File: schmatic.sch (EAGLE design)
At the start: 18 parts, among them SW1 SWITCH-SMD-EVQP-P2602W

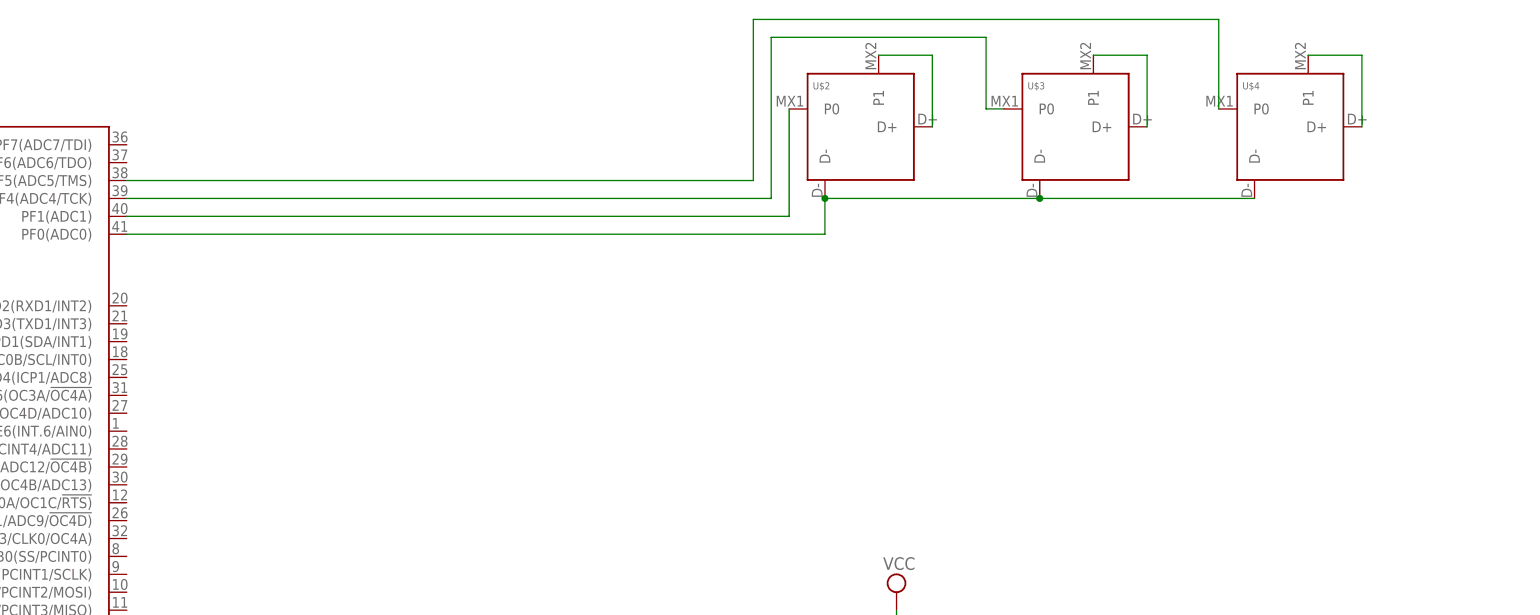
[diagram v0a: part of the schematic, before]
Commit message: updated based off feedback, included extra osh screenshot
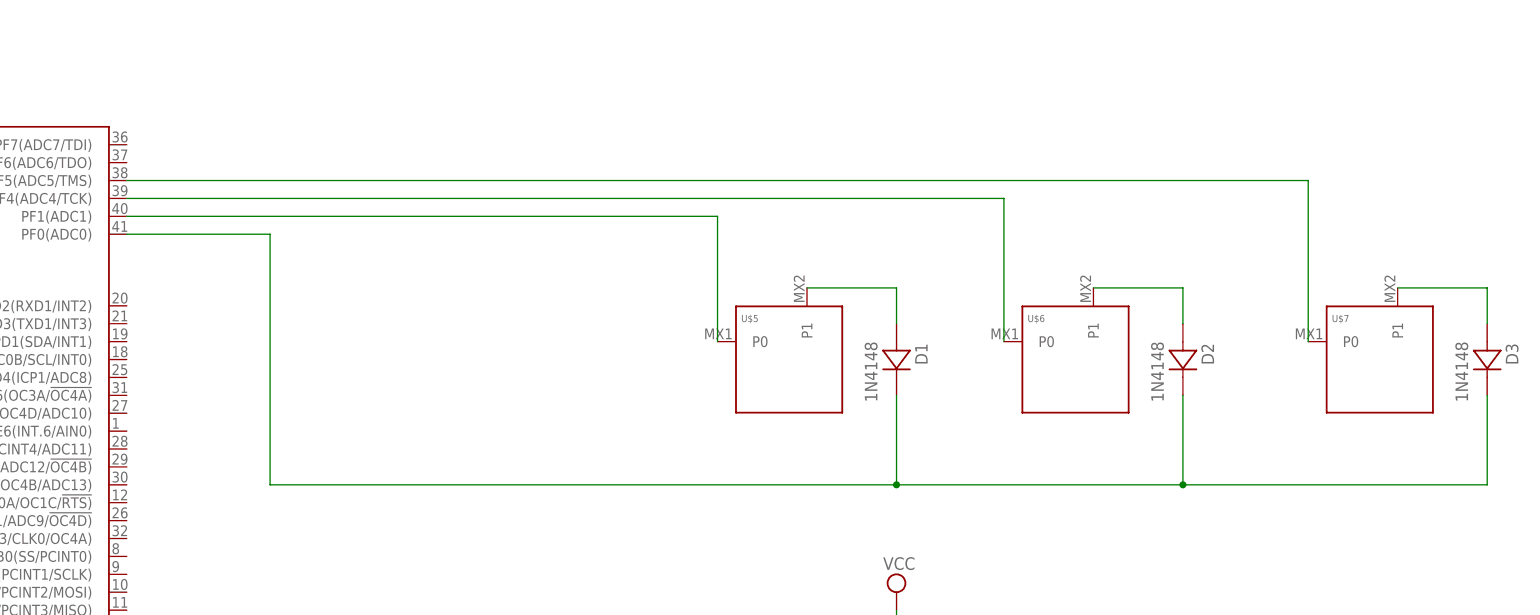
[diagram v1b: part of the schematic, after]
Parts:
- removed U$2, U$3, U$4: KEYSWITCH-DIODE-MX-1U-DIODE, Keyboard:KEYSWITCH-DIODE-MX-1U-DIODE
- added D1, D2, D3: 1N4148, Components:DIODE-DO-35
- added U$5, U$6, U$7: KEYSWITCH-PLAIN-MXHSPCB-1U, Keyboard:KEYSWITCH-PLAIN-MXHSPCB-1U
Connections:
- removed net N$11: U$3.D+, U$3.P1
- removed net N$12: U$4.D+, U$4.P1
- removed net N$16: U$1.PF5(ADC5/TMS), U$4.P0
- new net N$17: D1.A, U$5.P1
- new net N$18: D2.A, U$6.P1
- new net N$19: D3.A, U$7.P1
- net N$13: now also D1.C, D2.C, D3.C; no longer U$2.D-, U$3.D-, U$4.D-
- net N$14: now also U$5.P0; no longer U$2.P0
- net N$15: now also U$1.PF5(ADC5/TMS), U$7.P0; no longer U$1.PF4(ADC4/TCK), U$3.P0
- net N$9: now also U$1.PF4(ADC4/TCK), U$6.P0; no longer U$2.D+, U$2.P1
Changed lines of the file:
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@@
 <part name="SUPPLY6" library="supply2" library_urn="urn:adsk.eagle:library:372" deviceset="GND" device=""/>
 <part name="C8" library="Components" deviceset="CAPACITOR" device="-0402" value="1uF"/>
-<part name="U$2" library="Keyboard" deviceset="KEYSWITCH-DIODE" device="-MX-1U-DIODE"/>
-<part name="U$3" library="Keyboard" deviceset="KEYSWITCH-DIODE" device="-MX-1U-DIODE"/>
-<part name="U$4" library="Keyboard" deviceset="KEYSWITCH-DIODE" device="-MX-1U-DIODE"/>
 <part name="SUPPLY7" library="supply2" library_urn="urn:adsk.eagle:library:372" deviceset="GND" device=""/>
 <part name="SUPPLY8" library="supply2" library_urn="urn:adsk.eagle:library:372" deviceset="GND" device=""/>
@@
 <part name="SUPPLY14" library="supply2" library_urn="urn:adsk.eagle:library:372" deviceset="VCC" device=""/>
 <part name="SUPPLY15" library="supply2" library_urn="urn:adsk.eagle:library:372" deviceset="VCC" device=""/>
+<part name="U$5" library="Keyboard" deviceset="KEYSWITCH-PLAIN" device="-MXHSPCB-1U"/>
+<part name="U$6" library="Keyboard" deviceset="KEYSWITCH-PLAIN" device="-MXHSPCB-1U"/>
+<part name="U$7" library="Keyboard" deviceset="KEYSWITCH-PLAIN" device="-MXHSPCB-1U"/>
+<part name="D1" library="Components" deviceset="DIODE" device="-DO-35" value="1N4148"/>
+<part name="D2" library="Components" deviceset="DIODE" device="-DO-35" value="1N4148"/>
+<part name="D3" library="Components" deviceset="DIODE" device="-DO-35" value="1N4148"/>
 </parts>
 <sheets>
@@
 <attribute name="VALUE" x="77.216" y="86.106" size="1.778" layer="96" align="top-left"/>
 </instance>
-<instance part="U$2" gate="G$1" x="259.08" y="106.68" smashed="yes">
-<attribute name="NAME" x="252.27" y="111.998" size="1" layer="95"/>
-</instance>
-<instance part="U$3" gate="G$1" x="289.56" y="106.68" smashed="yes">
-<attribute name="NAME" x="282.75" y="111.998" size="1" layer="95"/>
-</instance>
-<instance part="U$4" gate="G$1" x="320.04" y="106.68" smashed="yes">
-<attribute name="NAME" x="313.23" y="111.998" size="1" layer="95"/>
-</instance>
 <instance part="SUPPLY7" gate="GND" x="93.98" y="38.1" smashed="yes" rot="R270">
 <attribute name="VALUE" x="90.805" y="40.005" size="1.778" layer="96" rot="R270"/>
@@
 <instance part="SUPPLY15" gate="G$1" x="93.98" y="91.44" smashed="yes" rot="R90">
 <attribute name="VALUE" x="90.805" y="89.535" size="1.778" layer="96" rot="R90"/>
+</instance>
+<instance part="U$5" gate="G$1" x="248.92" y="73.66" smashed="yes">
+<attribute name="NAME" x="242.11" y="78.978" size="1" layer="95"/>
+</instance>
+<instance part="U$6" gate="G$1" x="289.56" y="73.66" smashed="yes">
+<attribute name="NAME" x="282.75" y="78.978" size="1" layer="95"/>
+</instance>
+<instance part="U$7" gate="G$1" x="332.74" y="73.66" smashed="yes">
+<attribute name="NAME" x="325.93" y="78.978" size="1" layer="95"/>
+</instance>
+<instance part="D1" gate="D$1" x="264.16" y="73.66" smashed="yes" rot="R270">
+<attribute name="NAME" x="266.8016" y="75.9714" size="1.778" layer="95" rot="R270"/>
+<attribute name="VALUE" x="259.6642" y="76.2254" size="1.778" layer="96" rot="R270"/>
+</instance>
+<instance part="D2" gate="D$1" x="304.8" y="73.66" smashed="yes" rot="R270">
+<attribute name="NAME" x="307.4416" y="75.9714" size="1.778" layer="95" rot="R270"/>
+<attribute name="VALUE" x="300.3042" y="76.2254" size="1.778" layer="96" rot="R270"/>
+</instance>
+<instance part="D3" gate="D$1" x="347.98" y="73.66" smashed="yes" rot="R270">
+<attribute name="NAME" x="350.6216" y="75.9714" size="1.778" layer="95" rot="R270"/>
+<attribute name="VALUE" x="343.4842" y="76.2254" size="1.778" layer="96" rot="R270"/>
 </instance>
 </instances>
@@
 </segment>
 </net>
+<net name="N$13" class="0">
+<segment>
+<pinref part="U$1" gate="G$1" pin="PF0(ADC0)"/>
+<pinref part="D3" gate="D$1" pin="C"/>
+<wire x1="347.98" y1="68.58" x2="347.98" y2="55.88" width="0.1524" layer="91"/>
+<wire x1="347.98" y1="55.88" x2="304.8" y2="55.88" width="0.1524" layer="91"/>
+<wire x1="304.8" y1="55.88" x2="264.16" y2="55.88" width="0.1524" layer="91"/>
+<wire x1="264.16" y1="55.88" x2="175.26" y2="55.88" width="0.1524" layer="91"/>
+<wire x1="175.26" y1="55.88" x2="175.26" y2="91.44" width="0.1524" layer="91"/>
+<wire x1="175.26" y1="91.44" x2="154.94" y2="91.44" width="0.1524" layer="91"/>
+<pinref part="D2" gate="D$1" pin="C"/>
+<wire x1="304.8" y1="68.58" x2="304.8" y2="55.88" width="0.1524" layer="91"/>
+<junction x="304.8" y="55.88"/>
+<pinref part="D1" gate="D$1" pin="C"/>
+<wire x1="264.16" y1="68.58" x2="264.16" y2="55.88" width="0.1524" layer="91"/>
+<junction x="264.16" y="55.88"/>
+</segment>
+</net>
+<net name="N$17" class="0">
+<segment>
+<pinref part="U$5" gate="G$1" pin="P1"/>
+<pinref part="D1" gate="D$1" pin="A"/>
+<wire x1="251.46" y1="83.82" x2="264.16" y2="83.82" width="0.1524" layer="91"/>
+<wire x1="264.16" y1="83.82" x2="264.16" y2="78.74" width="0.1524" layer="91"/>
+</segment>
+</net>
+<net name="N$18" class="0">
+<segment>
+<pinref part="U$6" gate="G$1" pin="P1"/>
+<pinref part="D2" gate="D$1" pin="A"/>
+<wire x1="292.1" y1="83.82" x2="304.8" y2="83.82" width="0.1524" layer="91"/>
+<wire x1="304.8" y1="83.82" x2="304.8" y2="78.74" width="0.1524" layer="91"/>
+</segment>
+</net>
+<net name="N$19" class="0">
+<segment>
+<pinref part="U$7" gate="G$1" pin="P1"/>
+<pinref part="D3" gate="D$1" pin="A"/>
+<wire x1="335.28" y1="83.82" x2="347.98" y2="83.82" width="0.1524" layer="91"/>
+<wire x1="347.98" y1="83.82" x2="347.98" y2="78.74" width="0.1524" layer="91"/>
+</segment>
+</net>
+<net name="N$14" class="0">
+<segment>
+<pinref part="U$5" gate="G$1" pin="P0"/>
+<pinref part="U$1" gate="G$1" pin="PF1(ADC1)"/>
+<wire x1="238.76" y1="76.2" x2="238.76" y2="93.98" width="0.1524" layer="91"/>
+<wire x1="238.76" y1="93.98" x2="154.94" y2="93.98" width="0.1524" layer="91"/>
+</segment>
+</net>
 <net name="N$9" class="0">
 <segment>
-<pinref part="U$2" gate="G$1" pin="D+"/>
-<wire x1="269.24" y1="106.68" x2="269.24" y2="116.84" width="0.1524" layer="91"/>
-<pinref part="U$2" gate="G$1" pin="P1"/>
-<wire x1="269.24" y1="116.84" x2="261.62" y2="116.84" width="0.1524" layer="91"/>
-</segment>
-</net>
-<net name="N$11" class="0">
-<segment>
-<pinref part="U$3" gate="G$1" pin="D+"/>
-<pinref part="U$3" gate="G$1" pin="P1"/>
-<wire x1="299.72" y1="106.68" x2="299.72" y2="116.84" width="0.1524" layer="91"/>
-<wire x1="299.72" y1="116.84" x2="292.1" y2="116.84" width="0.1524" layer="91"/>
-</segment>
-</net>
-<net name="N$12" class="0">
-<segment>
-<pinref part="U$4" gate="G$1" pin="D+"/>
-<pinref part="U$4" gate="G$1" pin="P1"/>
-<wire x1="330.2" y1="106.68" x2="330.2" y2="116.84" width="0.1524" layer="91"/>
-<wire x1="330.2" y1="116.84" x2="322.58" y2="116.84" width="0.1524" layer="91"/>
-</segment>
-</net>
-<net name="N$13" class="0">
-<segment>
-<pinref part="U$2" gate="G$1" pin="D-"/>
-<pinref part="U$3" gate="G$1" pin="D-"/>
-<wire x1="254" y1="96.52" x2="284.48" y2="96.52" width="0.1524" layer="91"/>
-<pinref part="U$4" gate="G$1" pin="D-"/>
-<wire x1="284.48" y1="96.52" x2="314.96" y2="96.52" width="0.1524" layer="91"/>
-<junction x="284.48" y="96.52"/>
-<pinref part="U$1" gate="G$1" pin="PF0(ADC0)"/>
-<wire x1="254" y1="96.52" x2="254" y2="91.44" width="0.1524" layer="91"/>
-<wire x1="254" y1="91.44" x2="154.94" y2="91.44" width="0.1524" layer="91"/>
-<junction x="254" y="96.52"/>
-</segment>
-</net>
-<net name="N$14" class="0">
-<segment>
-<pinref part="U$2" gate="G$1" pin="P0"/>
-<pinref part="U$1" gate="G$1" pin="PF1(ADC1)"/>
-<wire x1="248.92" y1="109.22" x2="248.92" y2="93.98" width="0.1524" layer="91"/>
-<wire x1="248.92" y1="93.98" x2="154.94" y2="93.98" width="0.1524" layer="91"/>
+<pinref part="U$1" gate="G$1" pin="PF4(ADC4/TCK)"/>
+<pinref part="U$6" gate="G$1" pin="P0"/>
+<wire x1="154.94" y1="96.52" x2="279.4" y2="96.52" width="0.1524" layer="91"/>
+<wire x1="279.4" y1="96.52" x2="279.4" y2="76.2" width="0.1524" layer="91"/>
 </segment>
 </net>
 <net name="N$15" class="0">
 <segment>
-<pinref part="U$3" gate="G$1" pin="P0"/>
-<wire x1="279.4" y1="109.22" x2="276.86" y2="109.22" width="0.1524" layer="91"/>
-<wire x1="276.86" y1="109.22" x2="276.86" y2="119.38" width="0.1524" layer="91"/>
-<wire x1="276.86" y1="119.38" x2="246.38" y2="119.38" width="0.1524" layer="91"/>
-<wire x1="246.38" y1="119.38" x2="246.38" y2="96.52" width="0.1524" layer="91"/>
-<pinref part="U$1" gate="G$1" pin="PF4(ADC4/TCK)"/>
-<wire x1="246.38" y1="96.52" x2="154.94" y2="96.52" width="0.1524" layer="91"/>
-</segment>
-</net>
-<net name="N$16" class="0">
-<segment>
-<pinref part="U$4" gate="G$1" pin="P0"/>
-<wire x1="309.88" y1="109.22" x2="309.88" y2="121.92" width="0.1524" layer="91"/>
-<wire x1="309.88" y1="121.92" x2="243.84" y2="121.92" width="0.1524" layer="91"/>
-<wire x1="243.84" y1="121.92" x2="243.84" y2="99.06" width="0.1524" layer="91"/>
 <pinref part="U$1" gate="G$1" pin="PF5(ADC5/TMS)"/>
-<wire x1="243.84" y1="99.06" x2="154.94" y2="99.06" width="0.1524" layer="91"/>
-</segment>
-</net>
+<pinref part="U$7" gate="G$1" pin="P0"/>
+<wire x1="154.94" y1="99.06" x2="322.58" y2="99.06" width="0.1524" layer="91"/>
+<wire x1="322.58" y1="99.06" x2="322.58" y2="76.2" width="0.1524" layer="91"/>
+</segment>
+</net>
